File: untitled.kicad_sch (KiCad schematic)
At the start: 5 parts, among them J1 USB_B_Micro, P1 USB_C_Plug_USB2.0, U2 NCP1117-3.3_SOT223

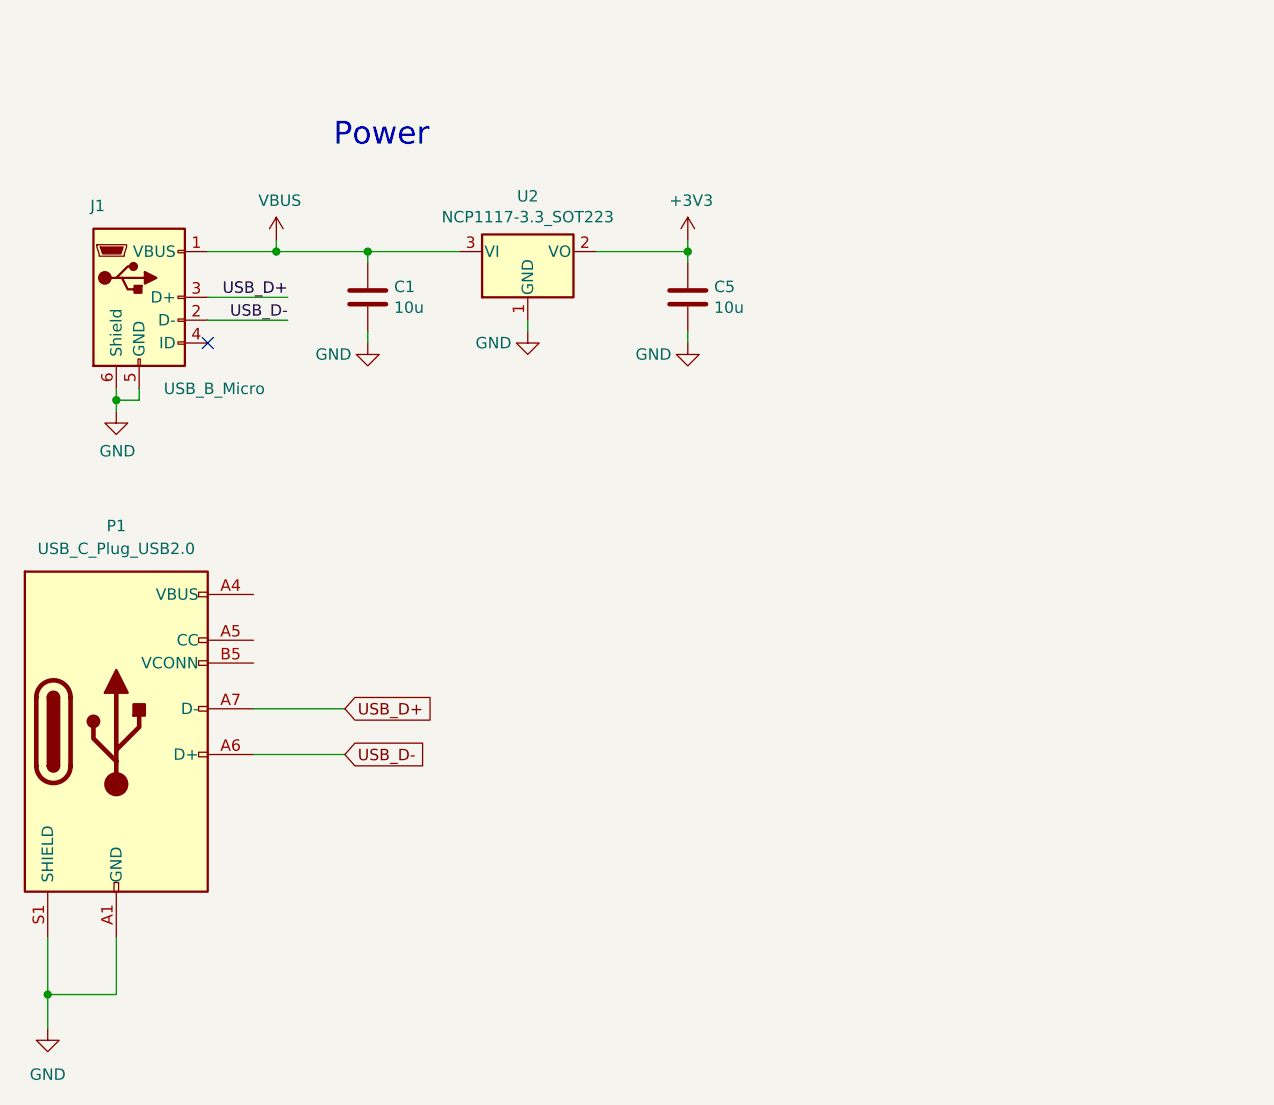
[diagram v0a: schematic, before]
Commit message: Add files via upload
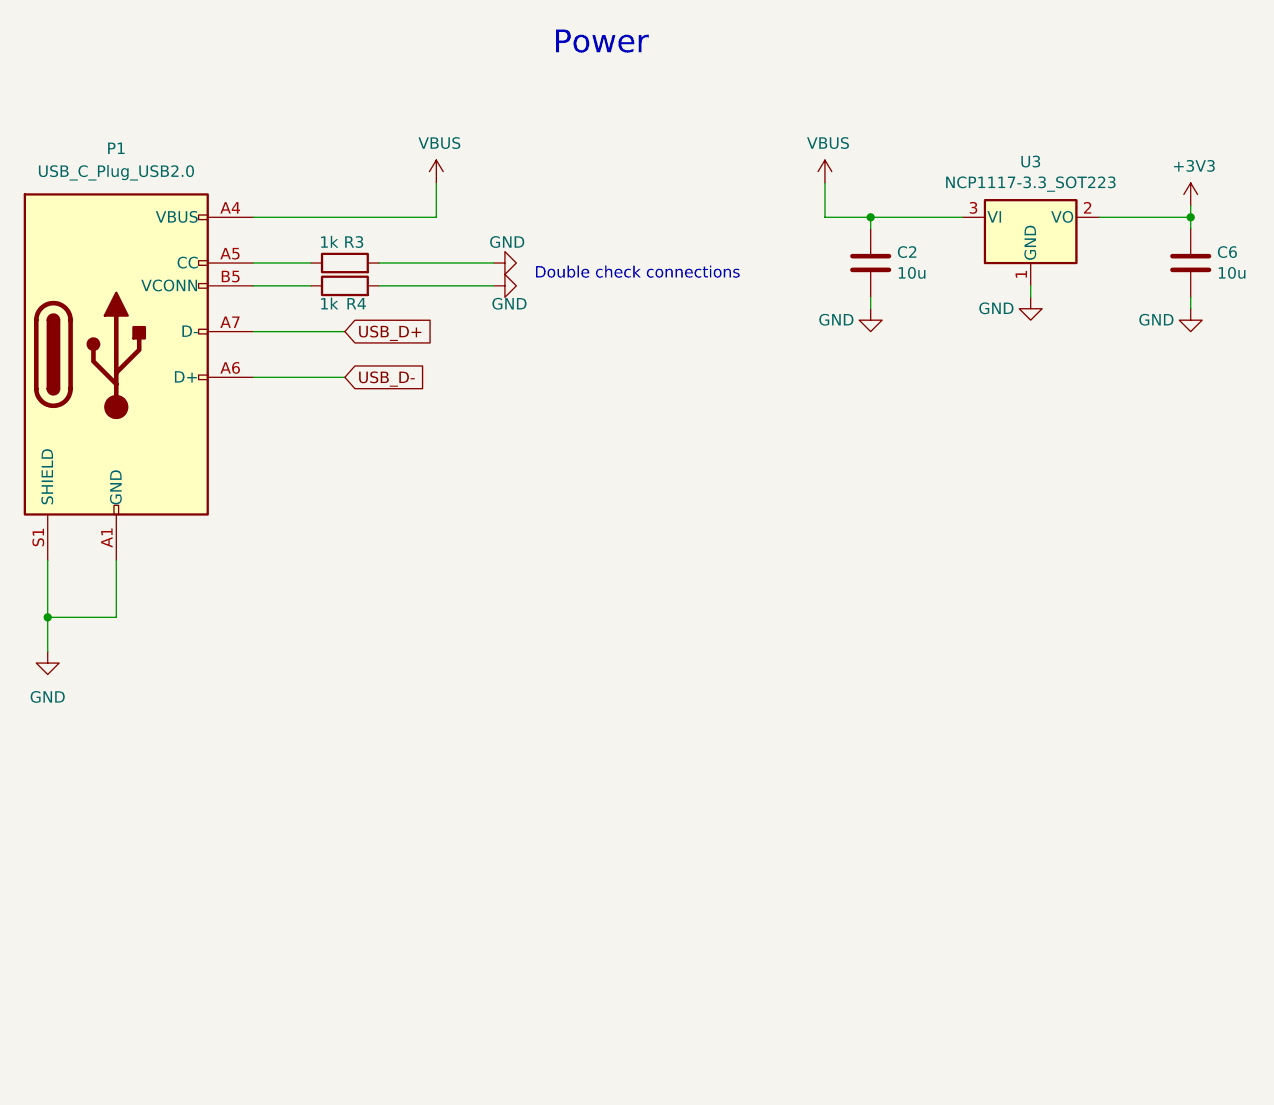
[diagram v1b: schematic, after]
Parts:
- removed C1, C5: 10u, Capacitor_SMD:C_0805_2012Metric, symbol Device:C
- removed J1: USB_B_Micro, Connector_USB:USB_Micro-B_Amphenol_10103594-0001LF_Horizontal, symbol Connector:USB_B_Micro
- removed U2: NCP1117-3.3_SOT223, Package_TO_SOT_SMD:SOT-223-3_TabPin2, symbol Regulator_Linear:NCP1117-3.3_SOT223
- added C2, C6: 10u, Capacitor_SMD:C_0805_2012Metric, symbol Device:C
- added R3, R4: 1k, symbol Device:R
- added U3: NCP1117-3.3_SOT223, Package_TO_SOT_SMD:SOT-223-3_TabPin2, symbol Regulator_Linear:NCP1117-3.3_SOT223
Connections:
- net +3V3: now also C6.1, U3.2 (VO)
- net GND: now also C2.2, C6.2, R3.2, R4.2, U3.1 (GND)
- net VBUS: now also P1.A4 (VBUS), P1.A9 (VBUS), P1.B4 (VBUS), P1.B9 (VBUS), C2.1, U3.3 (VI)
- net at P1.A5 (CC): now also R3.1
- net at P1.B5 (VCONN): now also R4.1
- no-connect marks 1 -> 0
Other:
- note added: "Double check connections"
